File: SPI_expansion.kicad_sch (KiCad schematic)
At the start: 5 parts, among them J1 Conn_02x05_Odd_Even

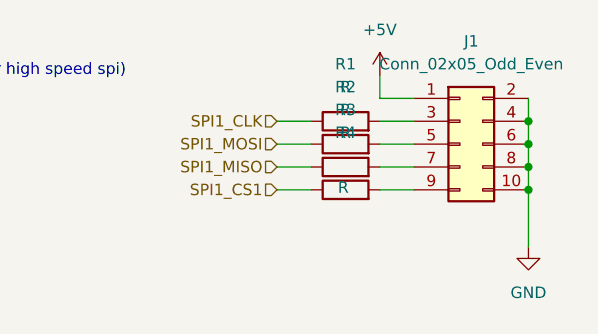
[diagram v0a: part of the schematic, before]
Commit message: Latest updates
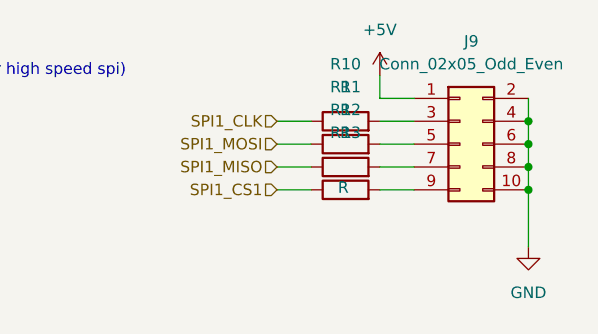
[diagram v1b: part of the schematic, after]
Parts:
- renumbered J1 to J9, R1 to R10, R2 to R11, R3 to R12, R4 to R13
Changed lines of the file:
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@@
 		(dnp no)
 		(fields_autoplaced yes)
-		(property "Reference" "#PWR06"
+		(property "Reference" "#PWR033"
 			(at 172.72 29.21 0)
 			(effects
@@
 			(project ""
 				(path "/38f33acd-ac87-4918-9c1f-d78977d10c9f/f251d033-7c4f-4f74-b0e8-105a8a585980"
-					(reference "#PWR06")
+					(reference "#PWR033")
 					(unit 1)
 				)
@@
 		(dnp no)
 		(fields_autoplaced yes)
-		(property "Reference" "R1"
+		(property "Reference" "R10"
 			(at 168.91 24.13 90)
 			(effects
@@
 			(project ""
 				(path "/38f33acd-ac87-4918-9c1f-d78977d10c9f/f251d033-7c4f-4f74-b0e8-105a8a585980"
-					(reference "R1")
+					(reference "R10")
 					(unit 1)
 				)
@@
 		(dnp no)
 		(fields_autoplaced yes)
-		(property "Reference" "R2"
+		(property "Reference" "R11"
 			(at 168.91 26.67 90)
 			(effects
@@
 			(project "OhWare"
 				(path "/38f33acd-ac87-4918-9c1f-d78977d10c9f/f251d033-7c4f-4f74-b0e8-105a8a585980"
-					(reference "R2")
+					(reference "R11")
 					(unit 1)
 				)
@@
 		(dnp no)
 		(fields_autoplaced yes)
-		(property "Reference" "J1"
+		(property "Reference" "J9"
 			(at 182.88 21.59 0)
 			(effects
@@
 			(project ""
 				(path "/38f33acd-ac87-4918-9c1f-d78977d10c9f/f251d033-7c4f-4f74-b0e8-105a8a585980"
-					(reference "J1")
+					(reference "J9")
 					(unit 1)
 				)
@@
 		(on_board yes)
 		(dnp no)
-		(property "Reference" "R4"
+		(property "Reference" "R13"
 			(at 168.91 31.75 90)
 			(effects
@@
 			(project "OhWare"
 				(path "/38f33acd-ac87-4918-9c1f-d78977d10c9f/f251d033-7c4f-4f74-b0e8-105a8a585980"
-					(reference "R4")
+					(reference "R13")
 					(unit 1)
 				)
@@
 		(dnp no)
 		(fields_autoplaced yes)
-		(property "Reference" "R3"
+		(property "Reference" "R12"
 			(at 168.91 29.21 90)
 			(effects
@@
 			(project "OhWare"
 				(path "/38f33acd-ac87-4918-9c1f-d78977d10c9f/f251d033-7c4f-4f74-b0e8-105a8a585980"
-					(reference "R3")
+					(reference "R12")
 					(unit 1)
 				)
@@
 		(dnp no)
 		(fields_autoplaced yes)
-		(property "Reference" "#PWR05"
+		(property "Reference" "#PWR034"
 			(at 189.23 50.8 0)
 			(effects
@@
 			(project ""
 				(path "/38f33acd-ac87-4918-9c1f-d78977d10c9f/f251d033-7c4f-4f74-b0e8-105a8a585980"
-					(reference "#PWR05")
-					(unit 1)
-				)
+					(reference "#PWR034")
+					(unit 1)
+				)
